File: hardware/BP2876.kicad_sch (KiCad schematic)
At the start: 18 parts, among them U101 BP2876

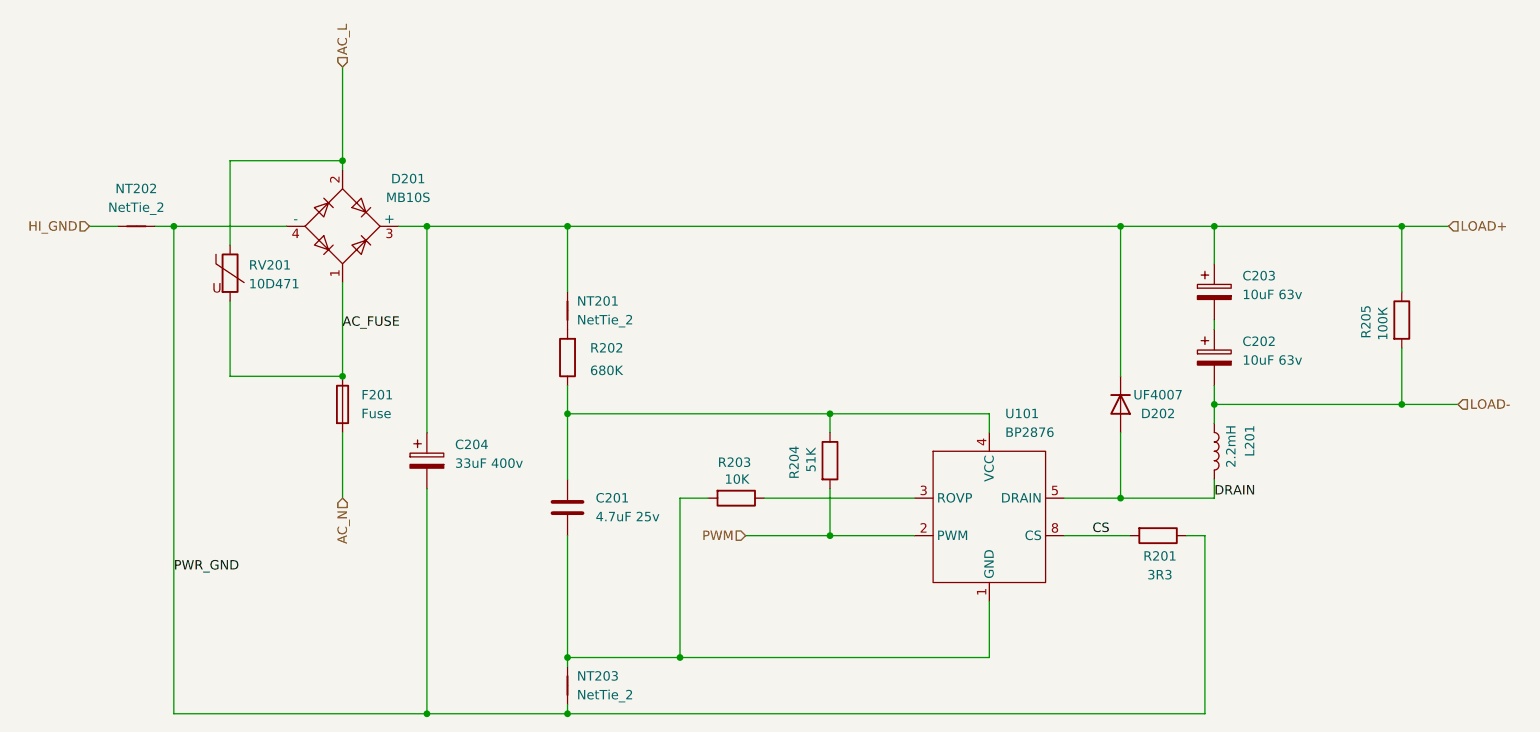
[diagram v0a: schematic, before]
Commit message: AC Input
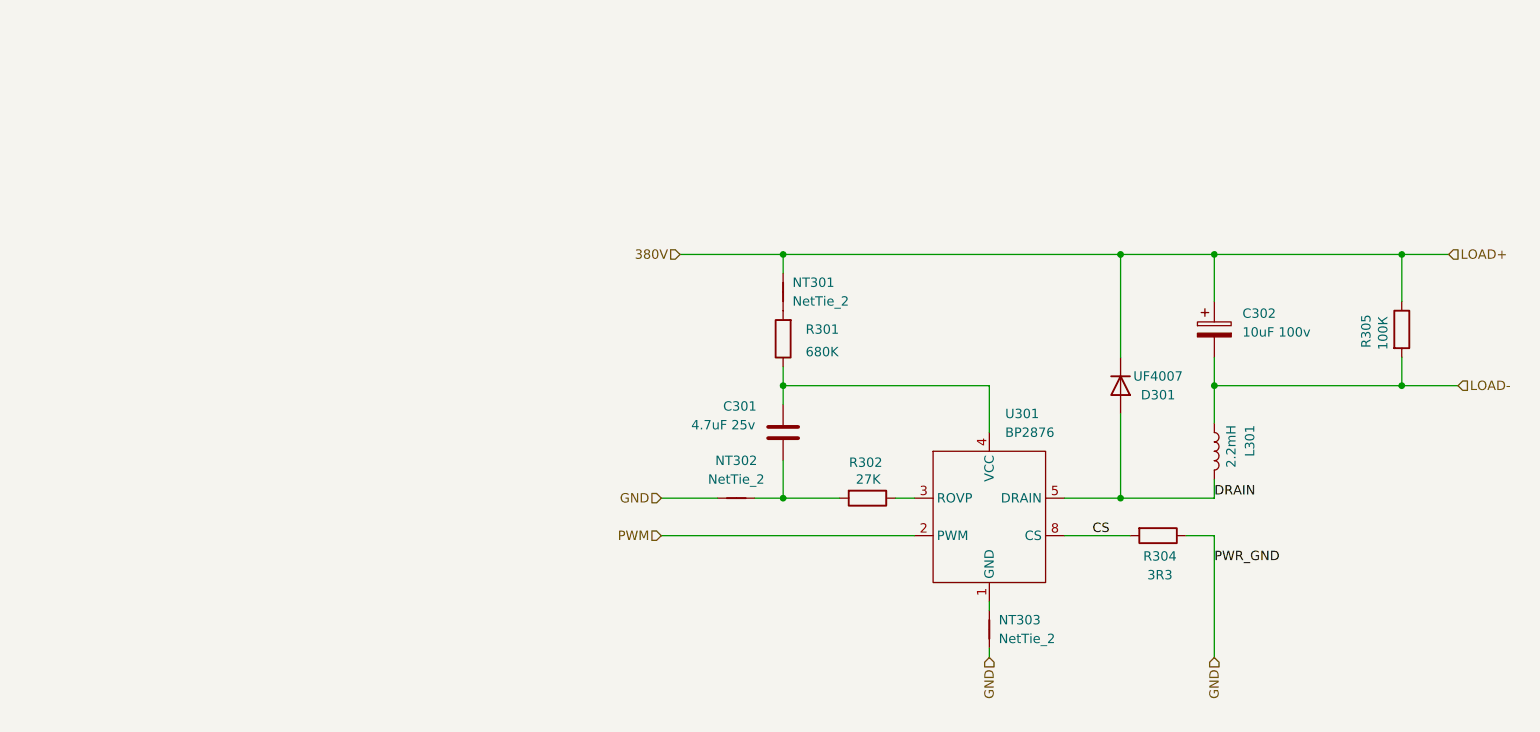
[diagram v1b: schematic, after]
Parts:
- removed C202: 10uF 63v, Capacitor_THT:CP_Radial_D5.0mm_P2.50mm, symbol Device:C_Polarized
- removed C204: 33uF 400v, Capacitor_THT:CP_Radial_D13.0mm_P5.00mm, symbol Device:C_Polarized
- removed D201: MB10S, Package_DIP:DIP-4_W7.62mm, symbol Diode_Bridge:MB6S
- removed F201: Fuse, Fuse:Fuseholder_Cylinder-5x20mm_Stelvio-Kontek_PTF78_Horizontal_Open, symbol Device:Fuse
- removed NT202: NetTie_2, NetTie:NetTie-2_SMD_Pad0.5mm, symbol Device:NetTie_2
- removed R204: 51K, Resistor_THT:R_Axial_DIN0207_L6.3mm_D2.5mm_P7.62mm_Horizontal, symbol Device:R
- removed RV201: 10D471, Varistor:RV_Disc_D12mm_W4.8mm_P7.5mm, symbol Device:Varistor
- added NT303: NetTie_2, NetTie:NetTie-2_SMD_Pad0.5mm, symbol Device:NetTie_2
- C302: renamed from C203; value 10uF 63v -> 10uF 100v; footprint Capacitor_THT:CP_Radial_D5.0mm_P2.50mm -> Capacitor_THT:CP_Radial_D6.3mm_P2.50mm
- R301: renamed from R202; footprint Resistor_THT:R_Axial_DIN0207_L6.3mm_D2.5mm_P7.62mm_Horizontal -> Resistor_THT:R_Axial_DIN0309_L9.0mm_D3.2mm_P12.70mm_Horizontal
- R302: renamed from R203; value 10K -> 27K
- renumbered C201 to C301, D202 to D301, L201 to L301, NT201 to NT301, NT203 to NT302, R201 to R304, R205 to R305, U101 to U301
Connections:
- net LOAD-: now also C302.2
- net at C301.2, R302.2: now also NT302.1; no longer NT302.2, U301.1 (GND)
- net LOAD+ renamed 380V
- net PWR_GND renamed GND
- net GND: now also NT302.2, NT303.1; no longer NT302.1
- new net: NT303.2, U301.1 (GND)
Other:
- moved on the sheet: C301, C302, D301, NT301, NT302, R301, R302, R305
